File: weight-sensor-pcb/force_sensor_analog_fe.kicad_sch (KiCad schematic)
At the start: 39 parts, among them IC2 INA333AIDGKR, IC3 INA333AIDGKR, IC4 INA333AIDGKR, IC5 INA333AIDGKR, J3 Conn_01x04_Socket, J5 Conn_01x04_Socket, J6 Conn_01x04_Socket, J7 Conn_01x04_Socket, U1 OPA333xxD, U2 OPA333xxD, U3 OPA333xxD, U5 OPA333xxD

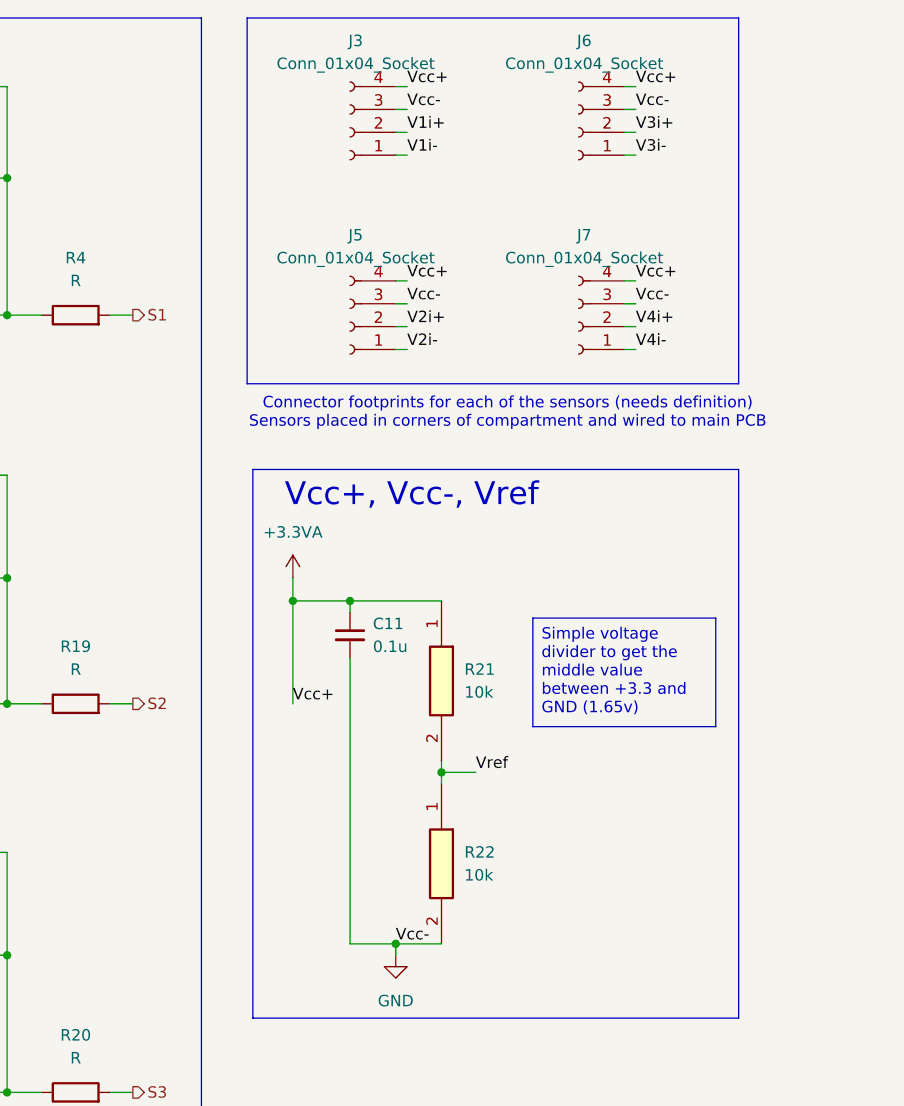
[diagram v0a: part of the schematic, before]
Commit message: started layout
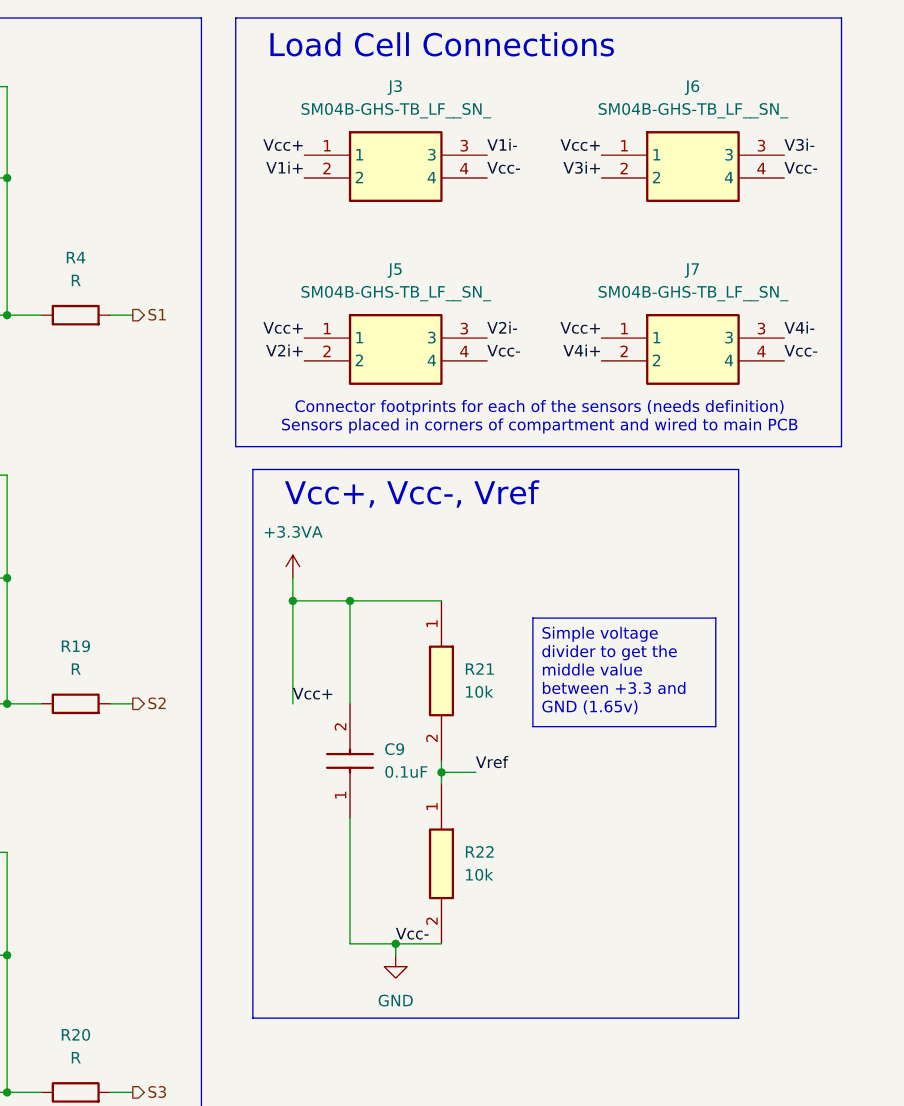
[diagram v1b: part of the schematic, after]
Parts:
- removed C11: 0.1u, symbol Device:C_Small
- removed J3, J5, J6, J7: Conn_01x04_Socket, symbol Connector:Conn_01x04_Socket
- added C9: 0.1uF, CAPC0603X33N, symbol Capstone:GRM033C71C104KE14D
- added J3, J5, J6, J7: SM04B-GHS-TB_LF__SN_, SM04B-GHS-TB, symbol Capstone:SM04B-GHS-TB_LF__SN_
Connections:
- net +3.3VA: now also C9.2, J3.1, J5.1, J6.1, J7.1
- net GND: now also C9.1, J3.4, J5.4, J6.4, J7.4
- net V1i+: now also J3.2
- net V1i-: now also J3.3
- net V2i+: now also J5.2
- net V2i-: now also J5.3
- net V3i+: now also J6.2
- net V3i-: now also J6.3
- net V4i+: now also J7.2
- net V4i-: now also J7.3
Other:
- note added: "Load Cell Connections"

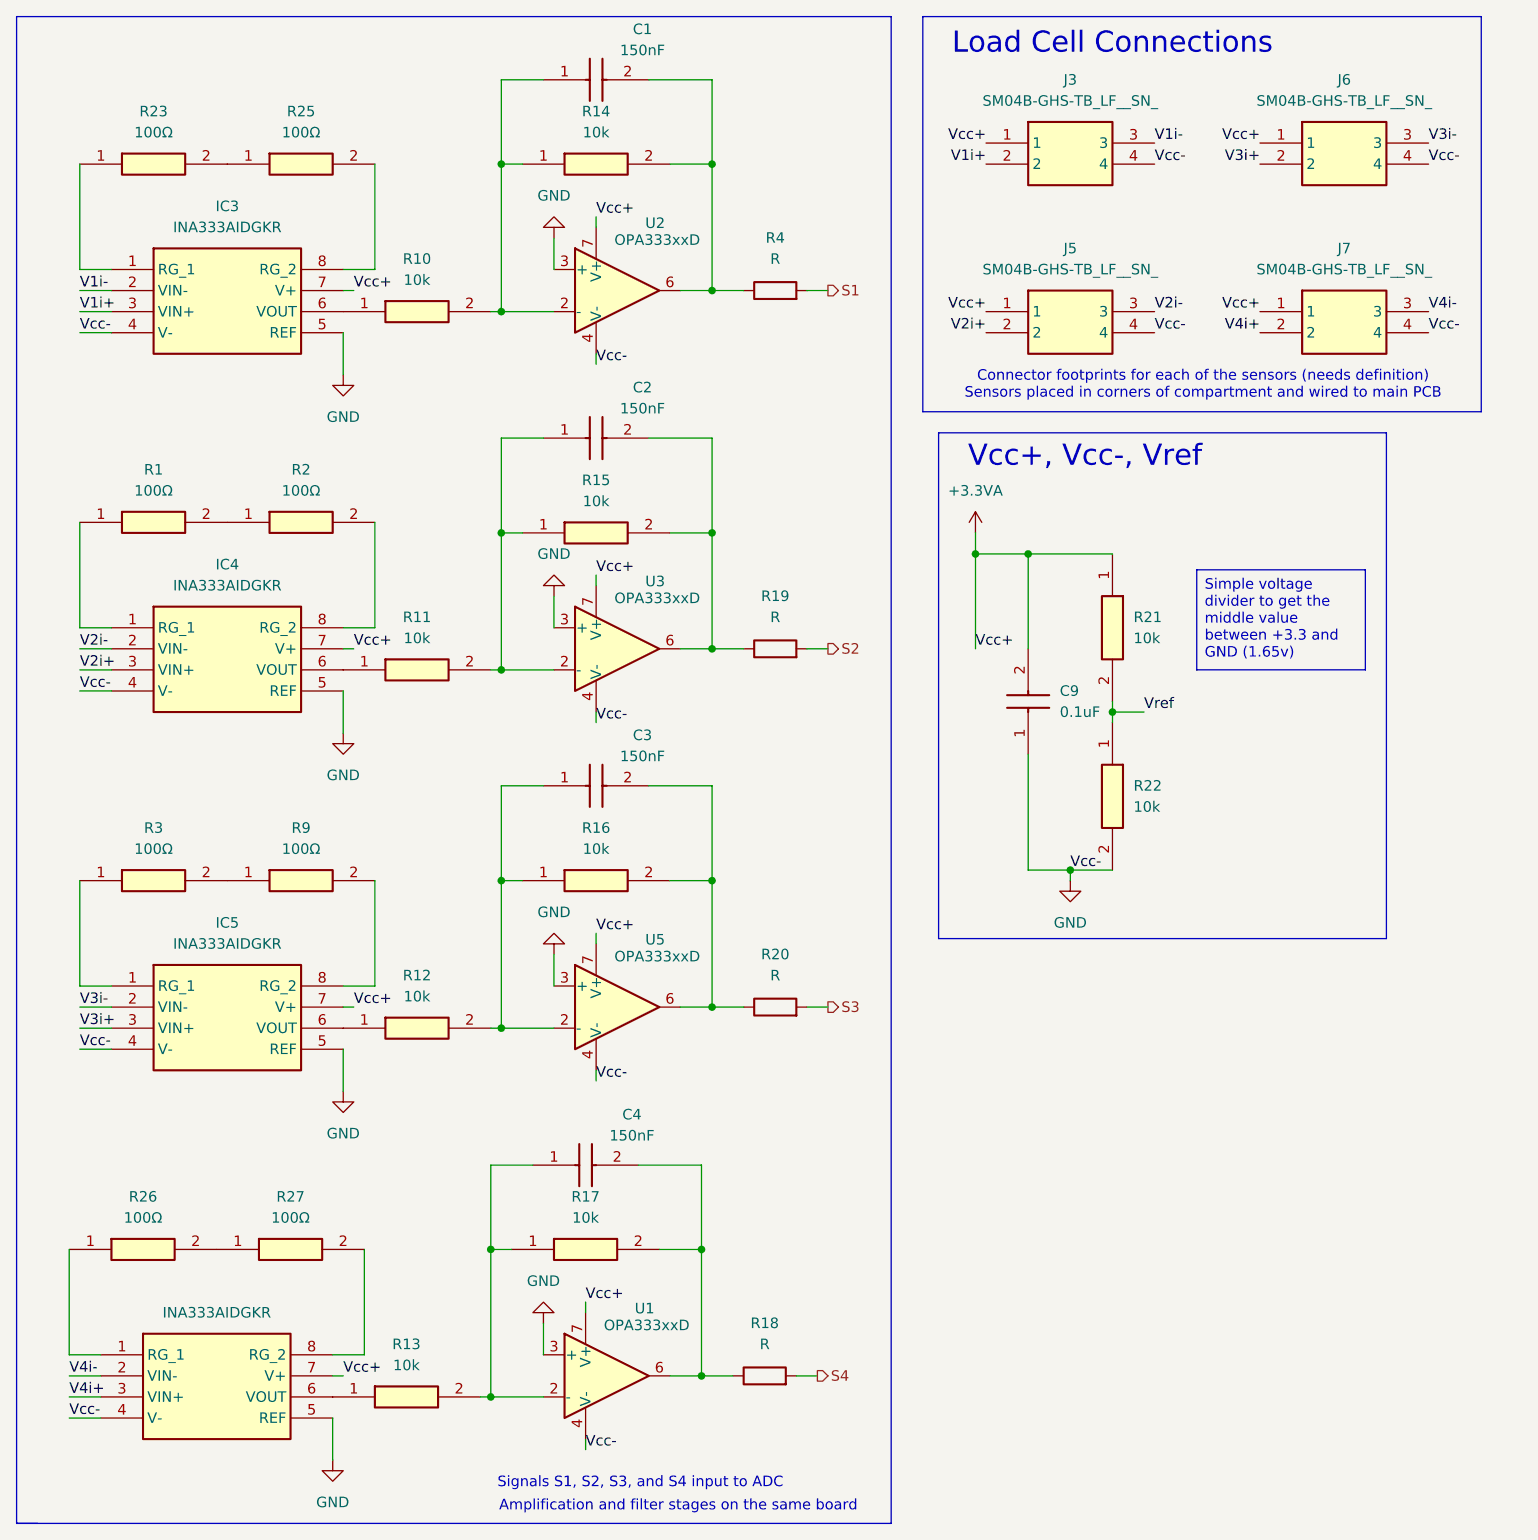
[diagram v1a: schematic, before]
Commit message: layout progress 1
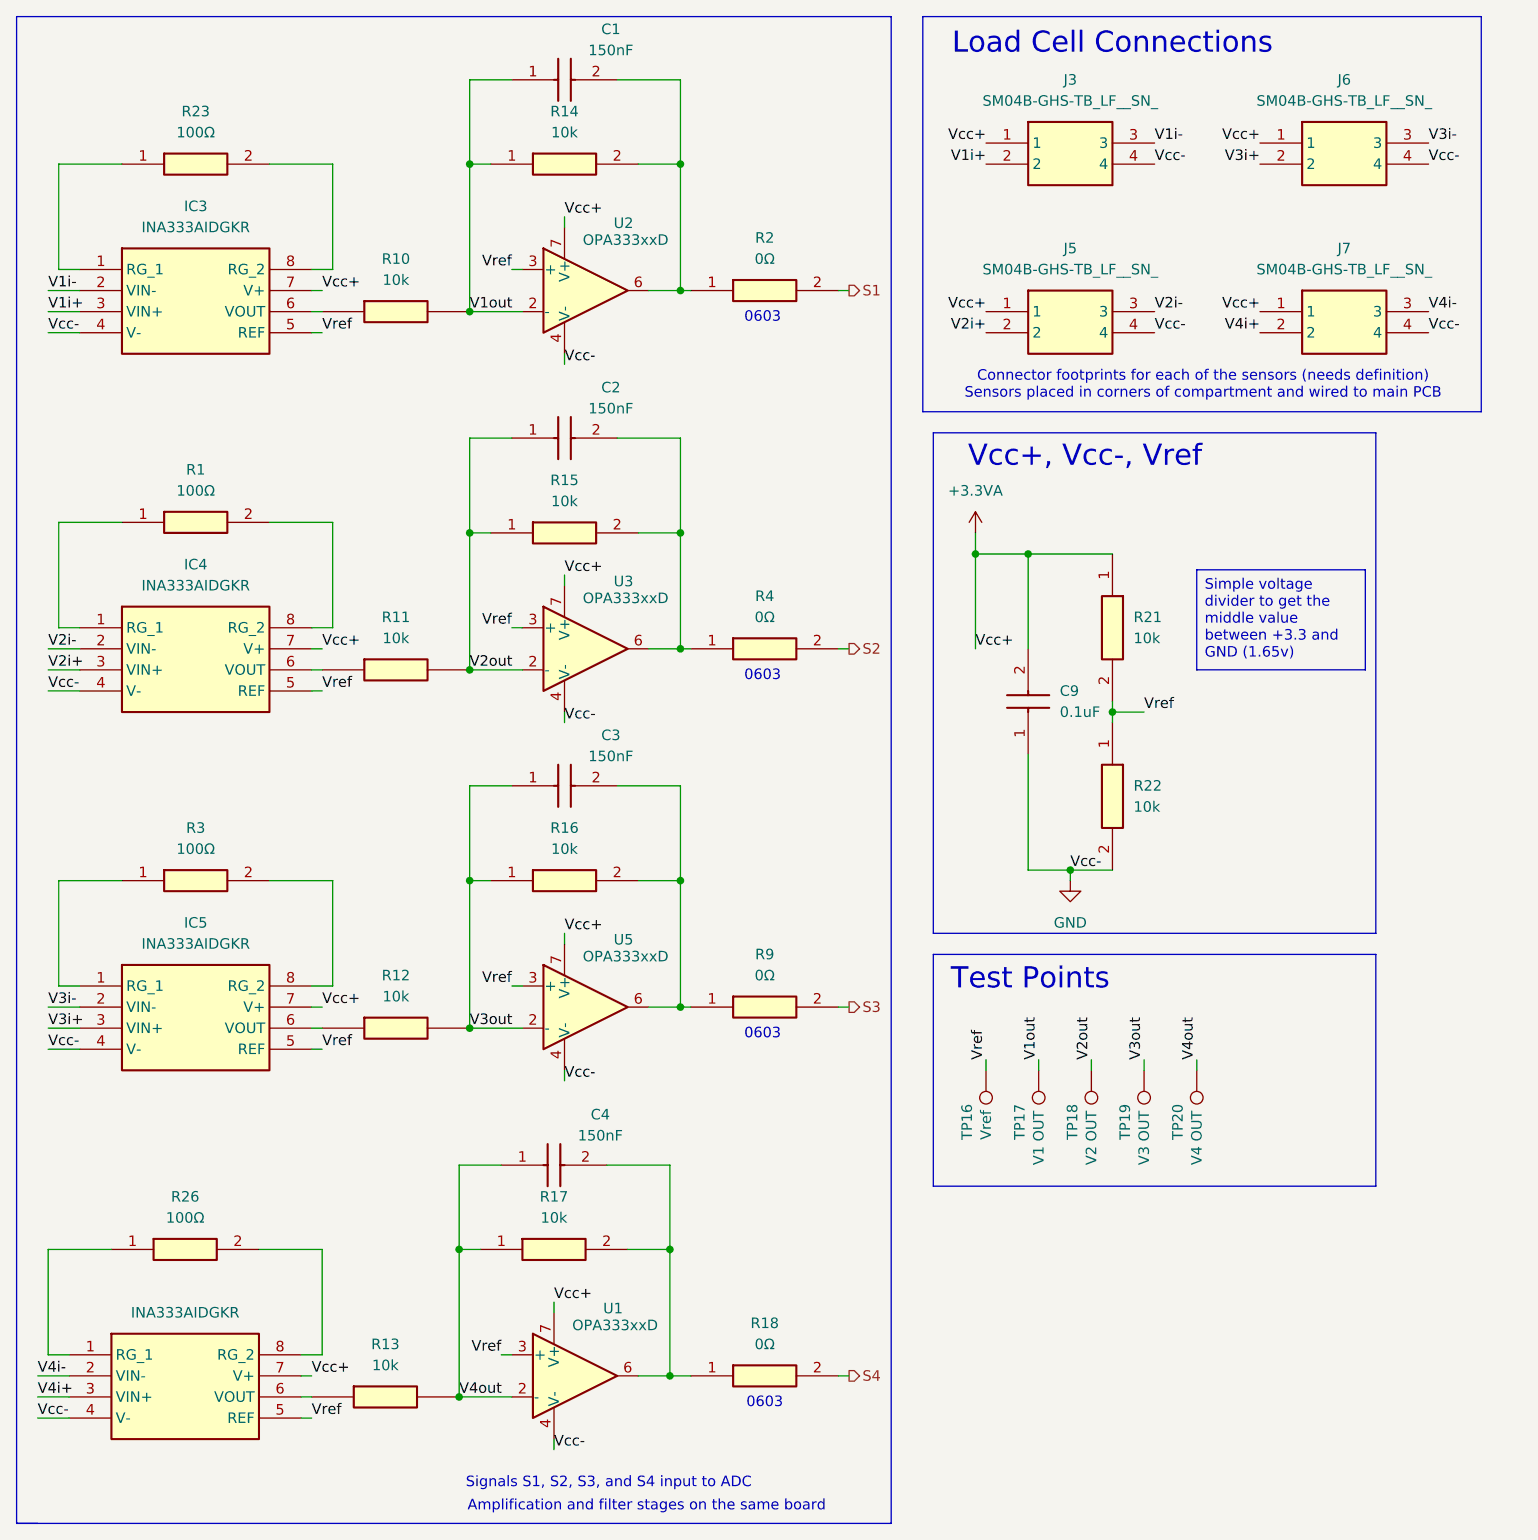
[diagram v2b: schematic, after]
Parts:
- removed R18, R19, R20, R4: R, symbol Device:R
- removed R2, R25, R27, R9: 100Ω, RESC1608X55N, symbol Capstone:RC0603FR-07100RL
- added R18, R2, R4, R9: 0Ω, RESC1608X55N, symbol Capstone:RC0603JR-070RL
- added TP16: Vref, TestPoint:TestPoint_Pad_D1.5mm, symbol Connector:TestPoint
- added TP17: V1 OUT, TestPoint:TestPoint_Pad_D1.5mm, symbol Connector:TestPoint
- added TP18: V2 OUT, TestPoint:TestPoint_Pad_D1.5mm, symbol Connector:TestPoint
- added TP19: V3 OUT, TestPoint:TestPoint_Pad_D1.5mm, symbol Connector:TestPoint
- added TP20: V4 OUT, TestPoint:TestPoint_Pad_D1.5mm, symbol Connector:TestPoint
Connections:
- net GND: no longer IC2.5 (REF), IC3.5 (REF), IC4.5 (REF), IC5.5 (REF), U1.3 (+), U2.3 (+), U3.3 (+), U5.3 (+)
- net S1: now also R2.2
- net S2: now also R4.2
- net S3: now also R9.2
- net S4: now also R18.2
- net Vref: now also IC2.5 (REF), IC3.5 (REF), IC4.5 (REF), IC5.5 (REF), U1.3 (+), U2.3 (+), U3.3 (+), U5.3 (+), TP16.1
- net V2out: now reaches C2.1, R11.2, R15.1, U3.2 (-)
- net V2out: now also TP18.1
- net at C2.2, R15.2, U3.6: now also R4.1
- net at R23.2: now also IC3.8 (RG_2)
- net at R26.2: now also IC2.8 (RG_2)
- net at R1.2: now also IC4.8 (RG_2)
- net at C3.2, R16.2, U5.6: now also R9.1
- net at C4.2, R17.2, U1.6: now also R18.1
- net at R3.2: now also IC5.8 (RG_2)
- net V1out: now reaches C1.1, R10.2, R14.1, U2.2 (-)
- net V1out: now also TP17.1
- net at C1.2, R14.2, U2.6: now also R2.1
- net V3out: now reaches C3.1, R12.2, R16.1, U5.2 (-)
- net V3out: now also TP19.1
- net V4out: now reaches C4.1, R13.2, R17.1, U1.2 (-)
- net V4out: now also TP20.1
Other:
- note added: "0603"
- note added: "Test Points"
- moved on the sheet: C1, C2, C3, C4, IC3, IC4, IC5, R1, R14, R15, R16, R17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

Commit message: Layout draft complete
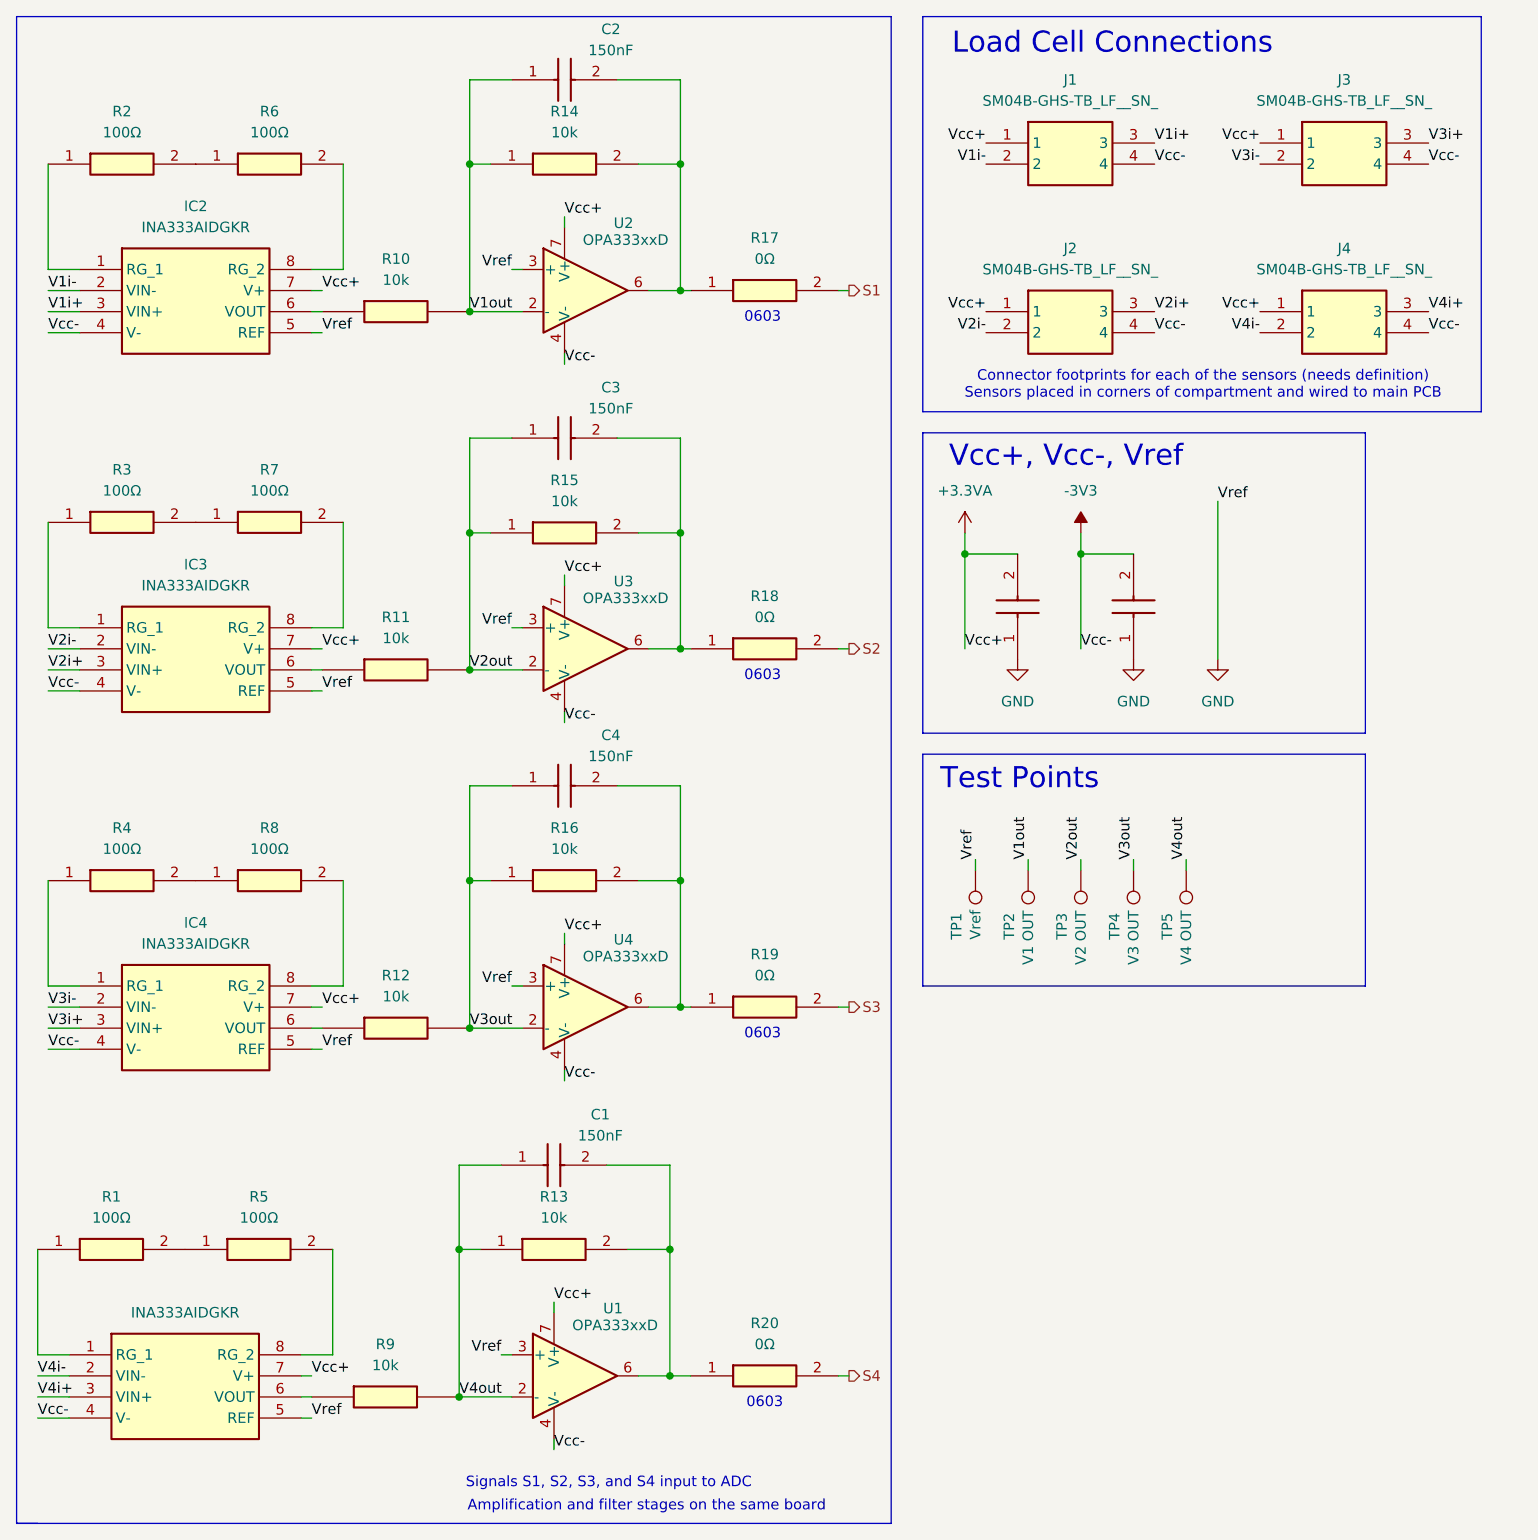
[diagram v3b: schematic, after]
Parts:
- removed R21, R22: 10k, RESC1608X55N, symbol Capstone:RMCF0603FT10K0
- added C6: 0.1uF, CAPC0603X33N, symbol Capstone:GRM033C71C104KE14D
- added R5, R6, R7, R8: 100Ω, RESC1608X55N, symbol Capstone:RC0603FR-07100RL
- renumbered C4 to C1, C1 to C2, C2 to C3, C3 to C4, C9 to C5, IC2 to IC1, IC3 to IC2, IC4 to IC3, IC5 to IC4, J3 to J1, J5 to J2, J6 to J3, J7 to J4, R26 to R1, R17 to R13, R2 to R17, R4 to R18, R9 to R19, R23 to R2, R18 to R20, R1 to R3, R3 to R4, R13 to R9, TP16 to TP1, TP17 to TP2, TP18 to TP3, TP19 to TP4, TP20 to TP5, U5 to U4
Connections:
- net Vref is gone; now on net GND: IC1.5 (REF), IC2.5 (REF), IC3.5 (REF), IC4.5 (REF), TP1.1, U1.3 (+), U2.3 (+), U3.3 (+), U4.3 (+)
- net GND: now also C6.1; no longer IC1.4 (V-), IC2.4 (V-), IC3.4 (V-), IC4.4 (V-), J1.4, J2.4, J3.4, J4.4, U1.4 (V-), U2.4 (V-), U3.4 (V-), U4.4 (V-)
- net V1i+: now also J1.3; no longer J1.2
- net V1i-: now also J1.2; no longer J1.3
- net V2i+: now also J2.3; no longer J2.2
- net V2i-: now also J2.2; no longer J2.3
- net V3i+: now also J3.3; no longer J3.2
- net V3i-: now also J3.2; no longer J3.3
- net V4i+: now also J4.3; no longer J4.2
- net V4i-: now also J4.2; no longer J4.3
- net at R2.2: now also R6.1; no longer IC2.8 (RG_2)
- net at IC1.8 (RG_2): now also R5.2; no longer R1.2
- net at R4.2: now also R8.1; no longer IC4.8 (RG_2)
- net at R3.2: now also R7.1; no longer IC3.8 (RG_2)
- new net: IC3.8 (RG_2), R7.2
- new net: R1.2, R5.1
- new net: IC2.8 (RG_2), R6.2
- new net: IC4.8 (RG_2), R8.2
- new net -3V3: C6.2, IC1.4 (V-), IC2.4 (V-), IC3.4 (V-), IC4.4 (V-), J1.4, J2.4, J3.4, J4.4, U1.4 (V-), U2.4 (V-), U3.4 (V-), U4.4 (V-)
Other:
- moved on the sheet: R1, R2, R3, R4, TP1, TP2, TP3, TP4, TP5
